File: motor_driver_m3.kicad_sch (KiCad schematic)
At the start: 31 parts, among them J10 Conn_01x01_Pin, J11 Conn_01x01_Pin, J12 Conn_01x01_Pin, M3 DRV8320SRTVR, Q13 NP80N06D6, Q14 NP80N06D6, Q15 NP80N06D6, Q16 NP80N06D6, Q17 NP80N06D6, Q18 NP80N06D6

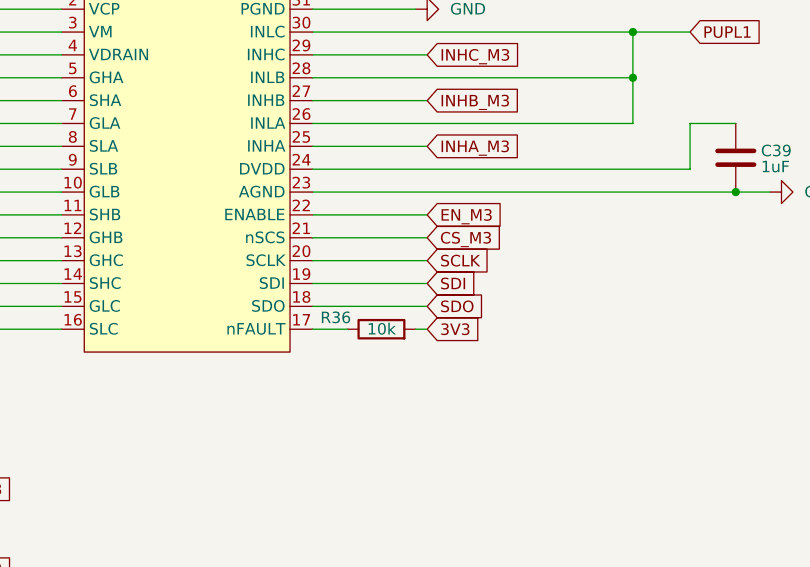
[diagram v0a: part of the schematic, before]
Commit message: ...
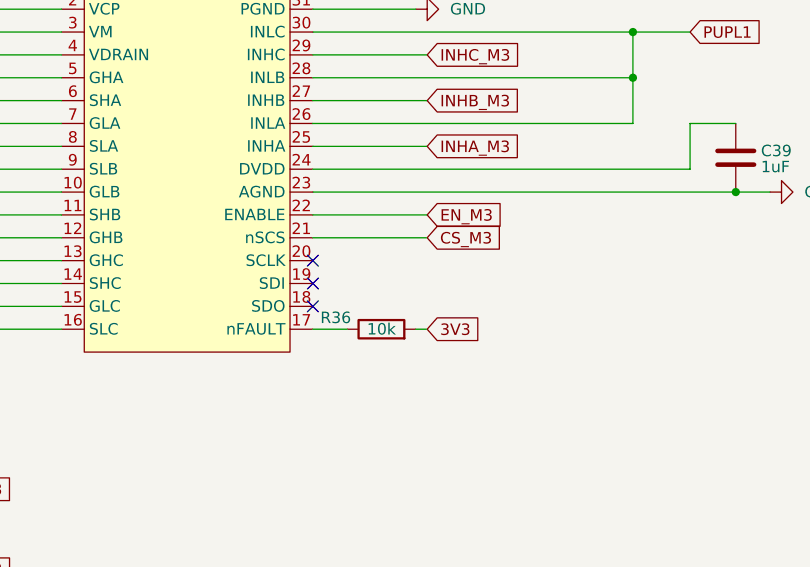
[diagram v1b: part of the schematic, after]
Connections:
- net SCLK: no longer names the net of M3.20 (SCLK)
- net SDI: no longer names the net of M3.19 (SDI)
- net SDO: no longer names the net of M3.18 (SDO)
- no-connect marks 0 -> 3
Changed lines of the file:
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@@
 		(color 0 0 0 0)
 	)
+	(no_connect
+		(at 92.71 80.01)
+	)
+	(no_connect
+		(at 92.71 74.93)
+	)
+	(no_connect
+		(at 92.71 77.47)
+	)
 	(wire
 		(pts
@@
 	(wire
 		(pts
-			(xy 105.41 74.93) (xy 92.71 74.93)
-		)
-		(stroke
-			(width 0)
-			(type default)
-		)
-	)
-	(wire
-		(pts
 			(xy 252.73 153.67) (xy 250.19 153.67)
 		)
@@
 	(wire
 		(pts
-			(xy 105.41 77.47) (xy 92.71 77.47)
-		)
-		(stroke
-			(width 0)
-			(type default)
-		)
-	)
-	(wire
-		(pts
 			(xy 252.73 52.07) (xy 250.19 52.07)
 		)
@@
 	(wire
 		(pts
-			(xy 92.71 80.01) (xy 105.41 80.01)
-		)
-		(stroke
-			(width 0)
-			(type default)
-		)
-	)
-	(wire
-		(pts
 			(xy 21.59 50.8) (xy 21.59 49.53)
 		)
@@
 		)
 	)
-	(global_label "SCLK"
-		(shape input)
-		(at 105.41 74.93 0)
-		(fields_autoplaced yes)
-		(effects
-			(font
-				(size 1.27 1.27)
-			)
-			(justify left)
-		)
-		(property "Intersheetrefs" "${INTERSHEET_REFS}"
-			(at 113.1728 74.93 0)
-			(effects
-				(font
-					(size 1.27 1.27)
-				)
-				(justify left)
-				(hide yes)
-			)
-		)
-	)
 	(global_label "SHB3"
 		(shape input)
@@
 		)
 	)
-	(global_label "SDI"
-		(shape input)
-		(at 105.41 77.47 0)
-		(fields_autoplaced yes)
-		(effects
-			(font
-				(size 1.27 1.27)
-			)
-			(justify left)
-		)
-		(property "Intersheetrefs" "${INTERSHEET_REFS}"
-			(at 111.4795 77.47 0)
-			(effects
-				(font
-					(size 1.27 1.27)
-				)
-				(justify left)
-				(hide yes)
-			)
-		)
-	)
 	(global_label "B+"
 		(shape input)
@@
 			(effects
 				(font
-					(size 1.27 1.27)
-				)
-				(justify left)
-				(hide yes)
-			)
-		)
-	)
-	(global_label "SDO"
-		(shape input)
-		(at 105.41 80.01 0)
-		(fields_autoplaced yes)
-		(effects
-			(font
-				(size 1.27 1.27)
-			)
-			(justify left)
-		)
-		(property "Intersheetrefs" "${INTERSHEET_REFS}"
-			(at 112.2052 80.01 0)
-			(effects
-				(font

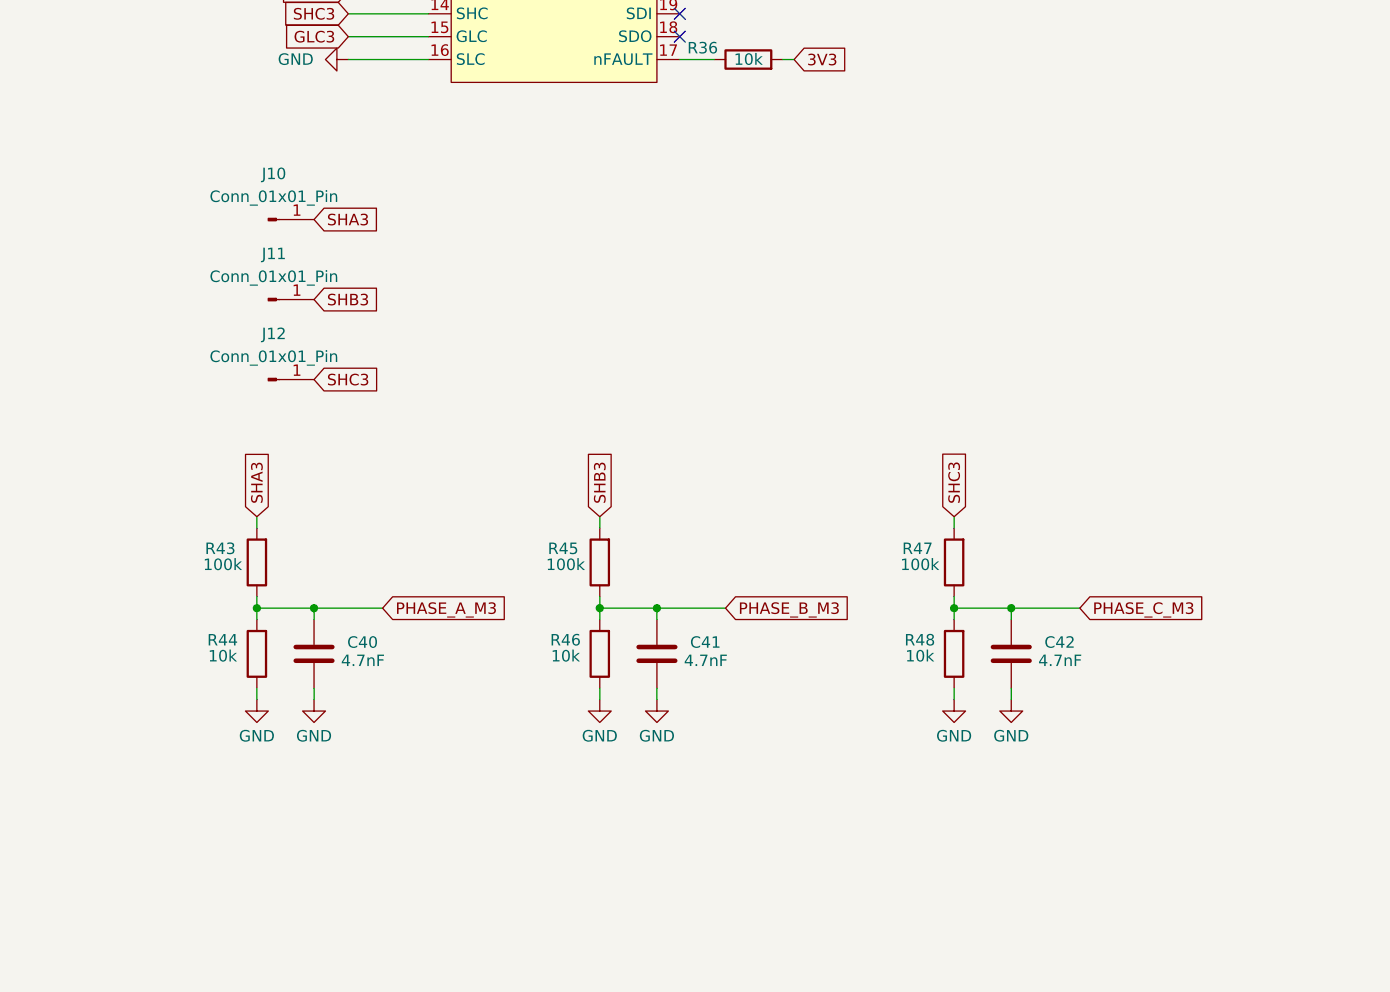
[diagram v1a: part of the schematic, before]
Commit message: ...
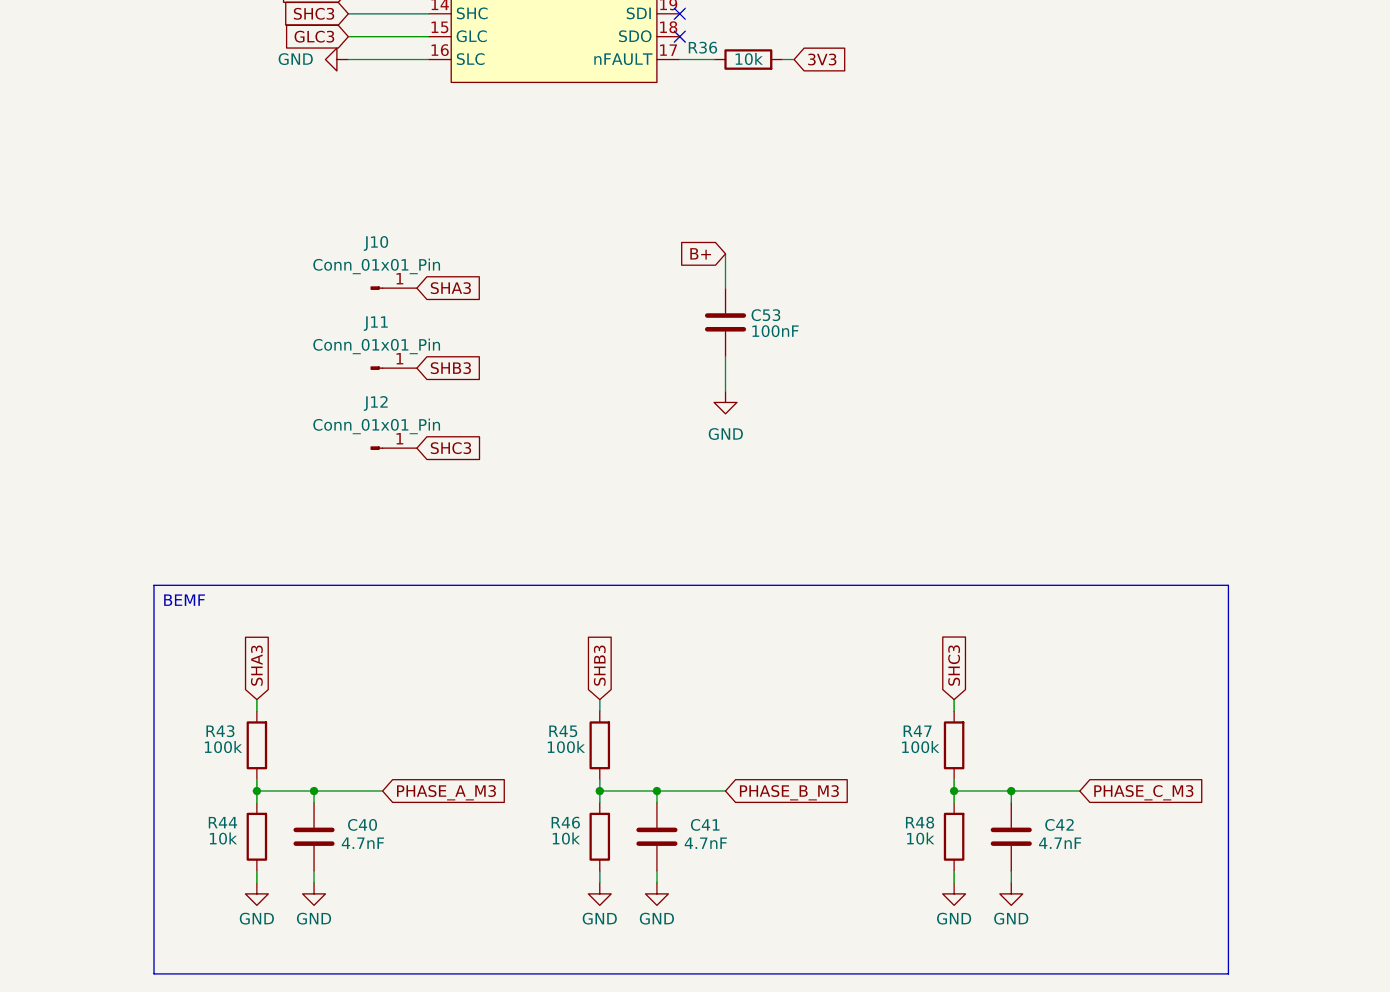
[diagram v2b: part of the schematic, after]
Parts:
- added C53: 100nF, easyeda2kicad:C0603, symbol Device:C
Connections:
- net B+: now also C53.1
- net GND: now also C53.2
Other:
- moved on the sheet: C40, C41, C42, J10, J11, J12, R43, R44, R45, R46, R47, R48

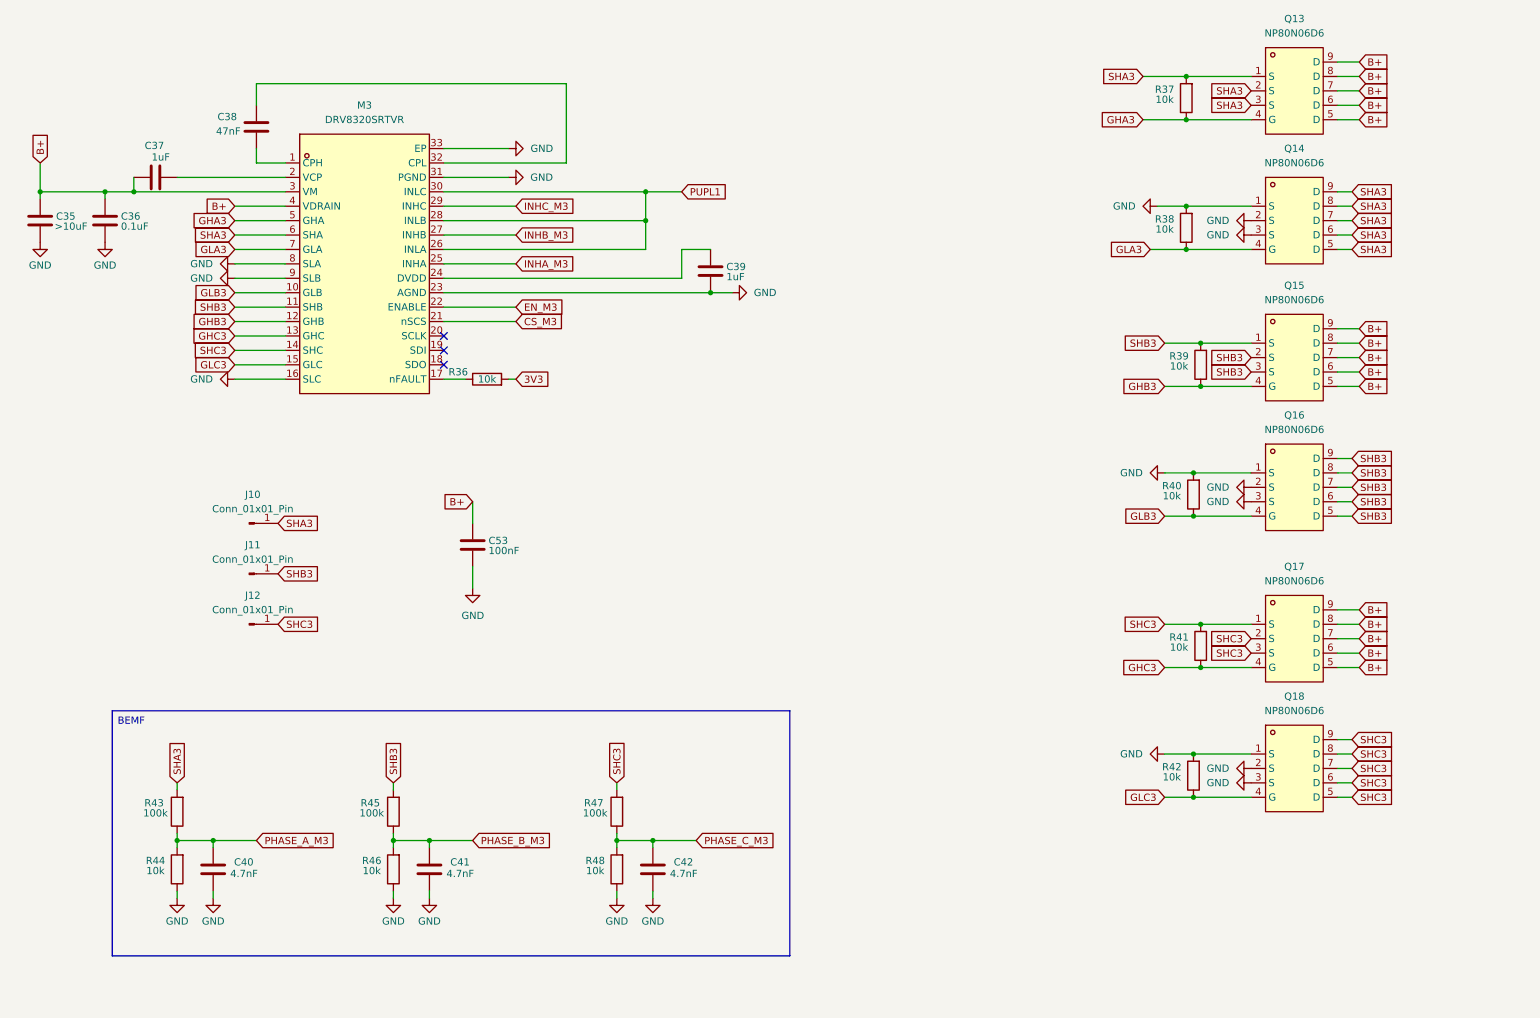
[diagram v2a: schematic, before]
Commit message: complete change in architecture,work in progress
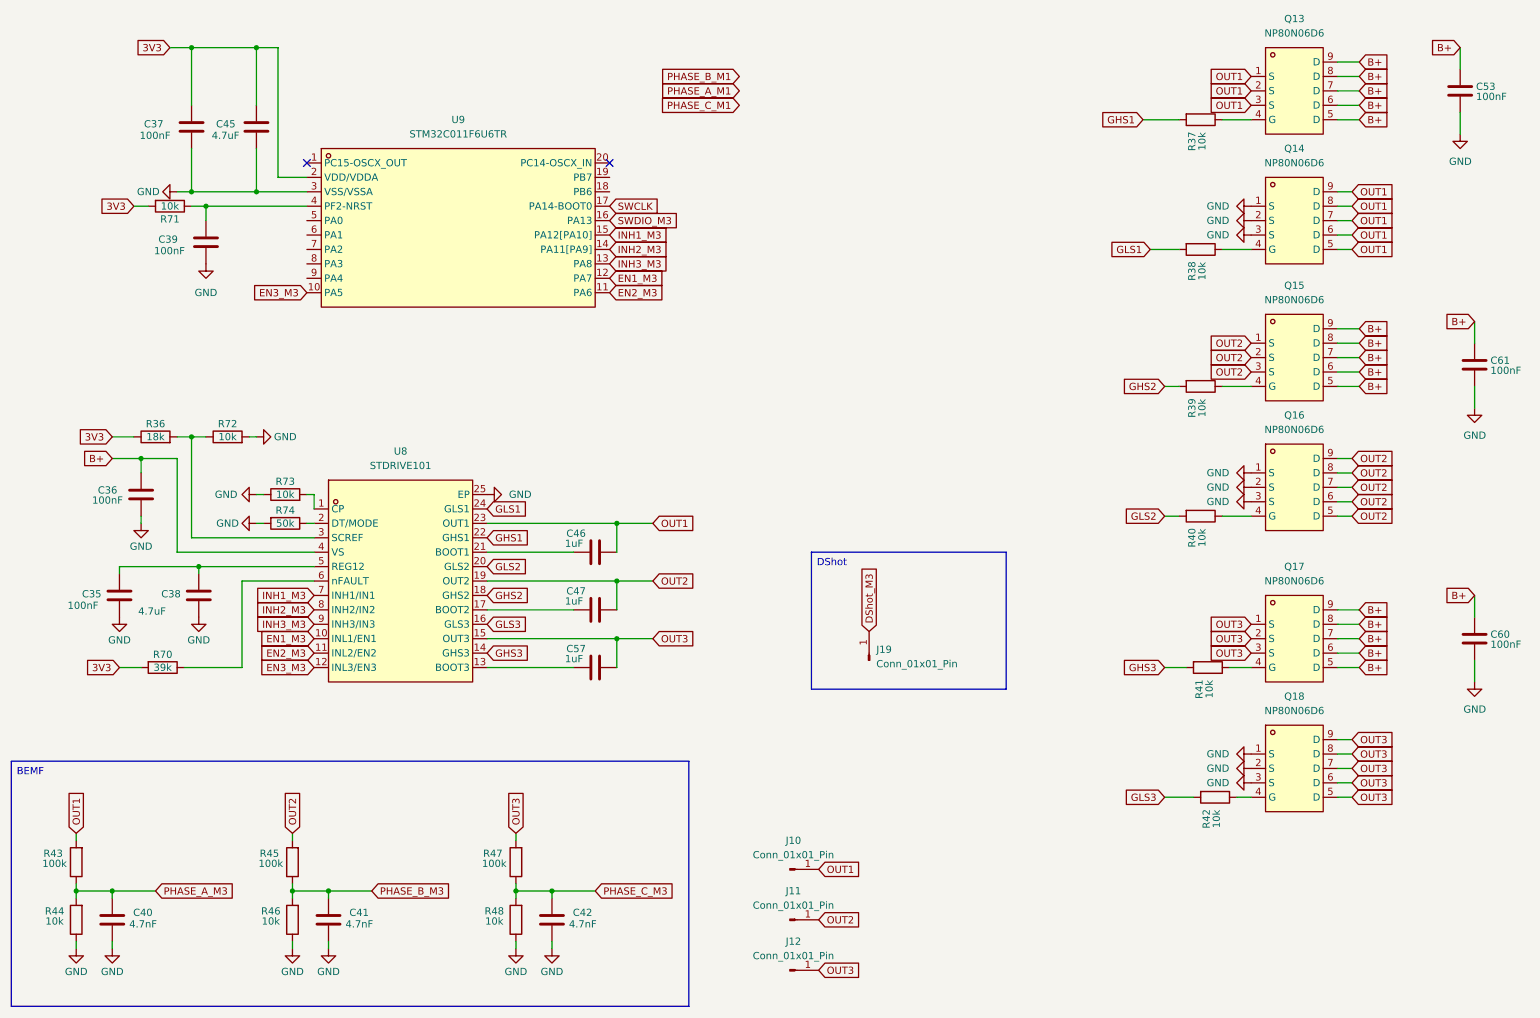
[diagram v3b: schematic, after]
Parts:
- removed M3: DRV8320SRTVR, easyeda2kicad:WQFN-32_L5.0-W5.0-P0.50-TL-EP3.5, symbol easyeda2kicad:DRV8320SRTVR
- added C45: 4.7uF, easyeda2kicad:C0402, symbol Device:C
- added C46, C47, C57: 1uF, easyeda2kicad:C0402, symbol Device:C
- added C60, C61: 100nF, easyeda2kicad:C0603, symbol Device:C
- added J19: Conn_01x01_Pin, deshan:Conn_1x1_small, symbol Connector:Conn_01x01_Pin
- added R70: 39k, easyeda2kicad:R0402, symbol Device:R
- added R71, R72, R73: 10k, easyeda2kicad:R0402, symbol Device:R
- added R74: 50k, easyeda2kicad:R0402, symbol Device:R
- added U8: STDRIVE101, easyeda2kicad:QFN-24_L4.0-W4.0-P0.50-BL-EP2.7, symbol easyeda2kicad:STDRIVE101
- added U9: STM32C011F6U6TR, easyeda2kicad:UFQFPN-20_L3.0-W3.0-P0.50-TL, symbol easyeda2kicad:STM32C011F6U6TR
- C35: value >10uF -> 100nF
- C36: value 0.1uF -> 100nF
- C37, C39: value 1uF -> 100nF; footprint easyeda2kicad:C0603 -> easyeda2kicad:C0402
- C38: value 47nF -> 4.7uF
- R36: value 10k -> 18k
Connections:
- net 3V3: now also C37.1, R36.1, C45.1, R70.2, R71.2, U9.2 (VDD/VDDA); no longer R36.2
- net B+: now also C60.1, C61.1, U8.4 (VS); no longer C35.1, C37.1
- net GND: now also C37.2, C38.2, C45.2, C60.2, C61.2, R72.2, R73.1, R74.2, U8.25 (EP), U9.3 (VSS/VSSA); no longer R38.2, R40.2, R42.2
- net at C38.1: now also C35.1, U8.5 (REG12)
- net at C39.1: now also R71.1, U9.4 (PF2-NRST)
- net GHA3: no longer names the net of Q13.4 (G), R37.1
- net GHB3: no longer names the net of Q15.4 (G), R39.1
- net GHC3: no longer names the net of Q17.4 (G), R41.1
- net GLA3: no longer names the net of Q14.4 (G), R38.1
- net GLB3: no longer names the net of Q16.4 (G), R40.1
- net GLC3: no longer names the net of Q18.4 (G), R42.1
- net SHA3 renamed OUT1
- net OUT1: now also C46.1, U8.23 (OUT1); no longer R37.2
- net SHB3 renamed OUT2
- net OUT2: now also C47.1, U8.19 (OUT2); no longer R39.2
- net SHC3 renamed OUT3
- net OUT3: now also C57.1, U8.15 (OUT3); no longer R41.2
- new net: R73.2, U8.1 (CP)
- new net: C57.2, U8.13 (BOOT3)
- new net: C47.2, U8.17 (BOOT2)
- new net: R74.1, U8.2 (DT/MODE)
- new net: C46.2, U8.21 (BOOT1)
- new net: R36.2, R72.1, U8.3 (SCREF)
- new net: R70.1, U8.6 (nFAULT)
- new net DShot_M3: J19.1 (Pin_1)
- new net EN1_M3: U8.10 (INL1/EN1), U9.12 (PA7)
- new net EN2_M3: U8.11 (INL2/EN2), U9.11 (PA6)
- new net EN3_M3: U8.12 (INL3/EN3), U9.10 (PA5)
- new net GHS1: R37.2, U8.22 (GHS1)
- new net GHS2: R39.2, U8.18 (GHS2)
- new net GHS3: R41.2, U8.14 (GHS3)
- new net GLS1: R38.2, U8.24 (GLS1)
- new net GLS2: R40.2, U8.20 (GLS2)
- new net GLS3: R42.2, U8.16 (GLS3)
- new net INH1_M3: U8.7 (INH1/IN1), U9.15 (PA12[PA10])
- new net INH2_M3: U8.8 (INH2/IN2), U9.14 (PA11[PA9])
- new net INH3_M3: U8.9 (INH3/IN3), U9.13 (PA8)
- new net SWCLK: U9.17 (PA14-BOOT0)
- new net SWDIO_M3: U9.16 (PA13)
- no-connect marks 3 -> 2
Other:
- moved on the sheet: C40, C41, C42, C53, J10, J11, J12, R37, R38, R39, R40, R41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
